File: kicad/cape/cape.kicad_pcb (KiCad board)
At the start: 2 copper layers, 86.4 x 54.6 mm, 17 parts, among them M1 HSR-2648CR, P1 BeagleBone_Black_Header, P2 BeagleBone_Black_Header, SW1 L101011_SPST, U1 L298, U2 BNO055, U3 BMP390, U4 S13V10FS

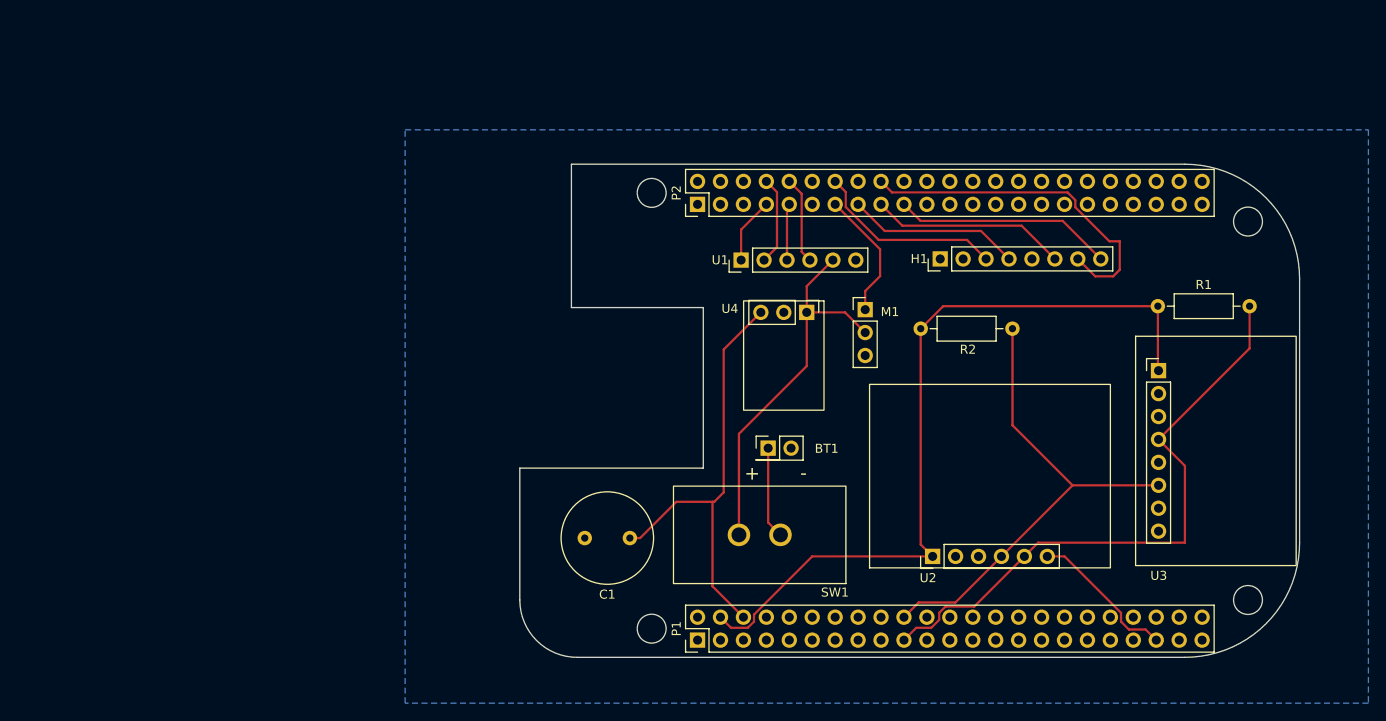
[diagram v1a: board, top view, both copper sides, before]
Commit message: Cape v 1.2
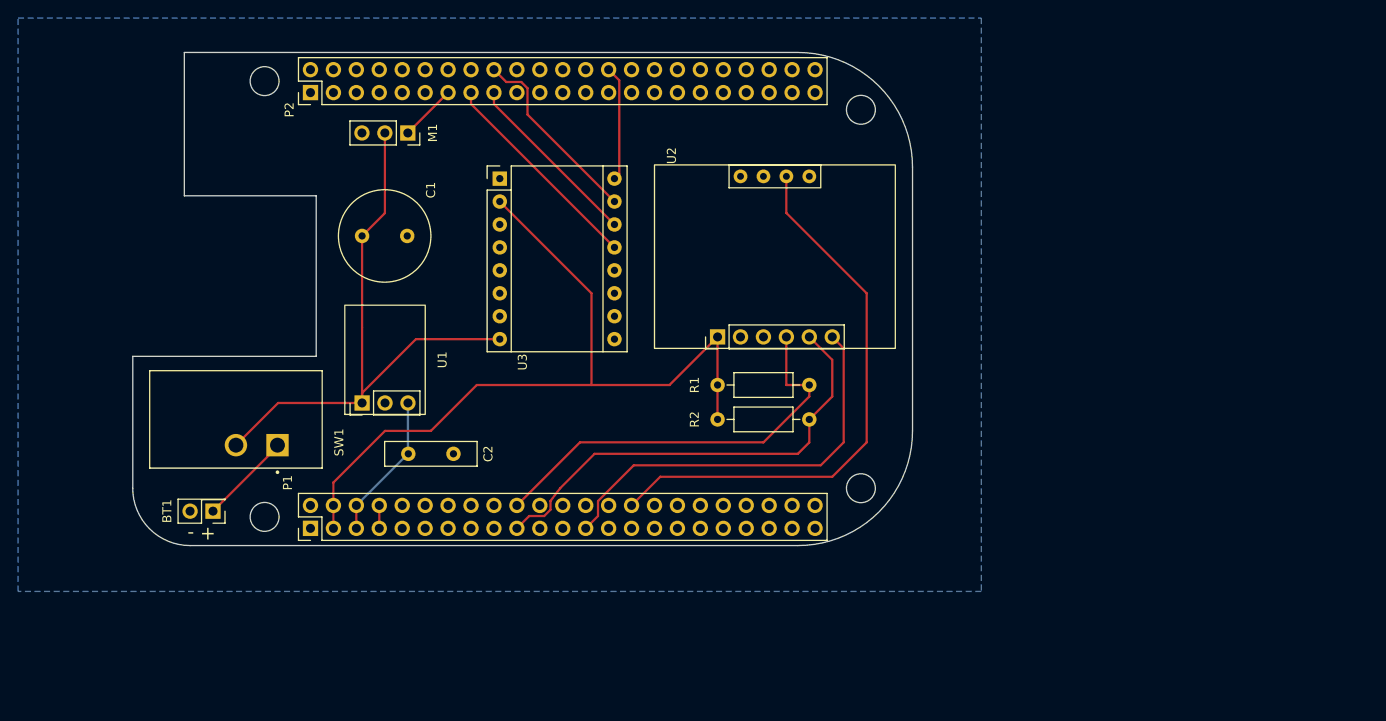
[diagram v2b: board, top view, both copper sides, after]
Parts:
- removed H1: GPIO_Breakout, Connector_PinHeader_2.54mm:PinHeader_1x08_P2.54mm_Vertical
- removed U4: S13V10FS, payload_footprint_library:S13V10F5
- added C2: 10 nF, Capacitor_THT:C_Disc_D10.0mm_W2.5mm_P5.00mm, F.Cu at (87.7, 77.5)
- C1: value 10 uF -> 100 uF
- M1: footprint Connector_PinHeader_2.54mm:PinHeader_1x03_P2.54mm_Vertical -> Connector_PinSocket_2.54mm:PinSocket_1x03_P2.54mm_Vertical
- SW1: footprint payload_footprint_library:SPST -> payload_footprint_library:SW_L101011MS02Q
- U1: value L298 -> S13V10F5; footprint Connector_PinHeader_2.54mm:PinHeader_1x06_P2.54mm_Vertical -> payload_footprint_library:S13V10F5
- U3: value BMP390 -> A4988; footprint payload_footprint_library:BMP390 -> payload_footprint_library:Pololu_Breakout-16_15.2x20.3mm
- moved U3 76.0 mm to (97.8, 47.0)
- moved BT1 61.9 mm to (66.0, 83.8), turned to 180 degrees
- moved SW1 59.4 mm to (68.6, 73.7)
- moved M1 54.3 mm to (87.6, 41.9), turned to -90 degrees
- moved R1 49.5 mm to (121.9, 69.8)
- moved U1 44.9 mm to (82.5, 71.8)
- moved C1 44.7 mm to (82.5, 53.3), turned to 0 degrees
- moved MH3 44.6 mm to (137.8, 39.4)
- moved MH4 44.6 mm to (137.8, 81.3)
- moved MH1 44.6 mm to (71.7, 36.2)
- moved MH2 44.6 mm to (71.7, 84.4)
- moved P1 44.6 mm to (76.8, 85.7)
- moved P2 44.6 mm to (76.8, 37.5)
- moved U2 34.0 mm to (121.9, 64.5)
- moved R2 24.6 mm to (121.9, 73.7)
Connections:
- net /GPIO[125] renamed /GPIO_115
- C1 pad 1: +5V -> /+7.4V
- P1 pad 30: /GPIO[122] -> /GPIO_112
- R1 pad 2: /I2C2.SCL -> /I2C2.SDA
- R2 pad 2: /I2C2.SDA -> /I2C2.SCL
- U1 pad 1: /GPIO[66] -> /+7.4V
- U1 pad 2: /GPIO[67] -> GNDD
- U1 pad 3: /GPIO[69] -> +5V
- U2 pad 6: /GPIO[20] -> /GPIO[117]
- U3 pad 1: +3.3V -> GNDD
- U3 pad 2: unconnected-(U3-Pad2) -> +3.3V
- U3 pad 3: GNDD -> unconnected-(U3-Pad3)
- U3 pad 4: /I2C2.SCL -> unconnected-(U3-Pad4)
- U3 pad 6: /I2C2.SDA -> unconnected-(U3-Pad6)
- U3 pad 7: unconnected-(U3-Pad7) -> GNDD
- U3 pad 8: unconnected-(U3-Pad8) -> /+7.4V
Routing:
- net /GPIO_112: track 0.00 -> 62.1 mm
- net /GPIO[117]: track 0.00 -> 45.7 mm
- net +5V: track 48.3 -> 16.3 mm
- net /GPIO[22]: track 24.3 -> 0.00 mm
- net /+7.4V: track 42.1 -> 65.7 mm
- net /GPIO[26]: track 21.2 -> 0.00 mm
- net /GPIO[65]: track 38.6 -> 21.1 mm
- net /I2C2.SCL: track 67.6 -> 50.8 mm
- net /GPIO[20]: track 16.5 -> 0.00 mm
- net /GPIO[61]: track 0.00 -> 12.8 mm
- net /GPIO[67]: track 9.79 -> 0.00 mm
- net /GPIO[68]: track 9.66 -> 0.00 mm
- net /GPIO[23]: track 14.4 -> 6.32 mm
- net /I2C2.SDA: track 54.3 -> 46.5 mm
- net /GPIO[66]: track 7.33 -> 0.00 mm
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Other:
- outline, holes or cut-outs redrawn
- board text added: "+ -"
- board text removed: "+"
- board text removed: "-"
